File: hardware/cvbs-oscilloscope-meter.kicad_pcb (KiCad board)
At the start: 2 copper layers, 49.5 x 99.7 mm, 40 parts, among them J1 Conn_Coaxial_Power, J2 Conn_Coaxial_Power, J3 Conn_Coaxial_Power, J4 Conn_Coaxial_Power, Q1 2N3906, Q2 2N3906, Q3 2N3904, Q4 2N3904, Q5 2N3904, Q6 2N3904, U1 LM1881, U4 AD8032

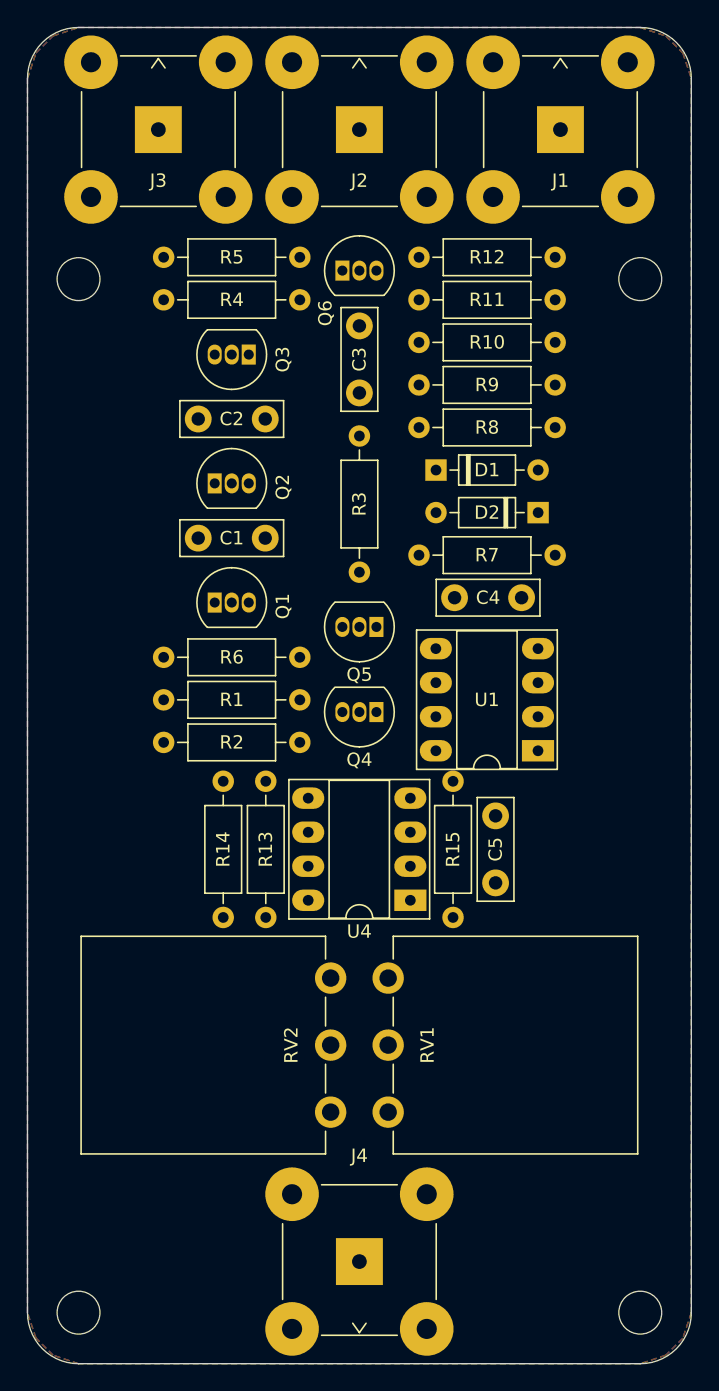
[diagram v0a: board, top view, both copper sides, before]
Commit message: Finished initial routing
Finished Routing - will need to check and revise
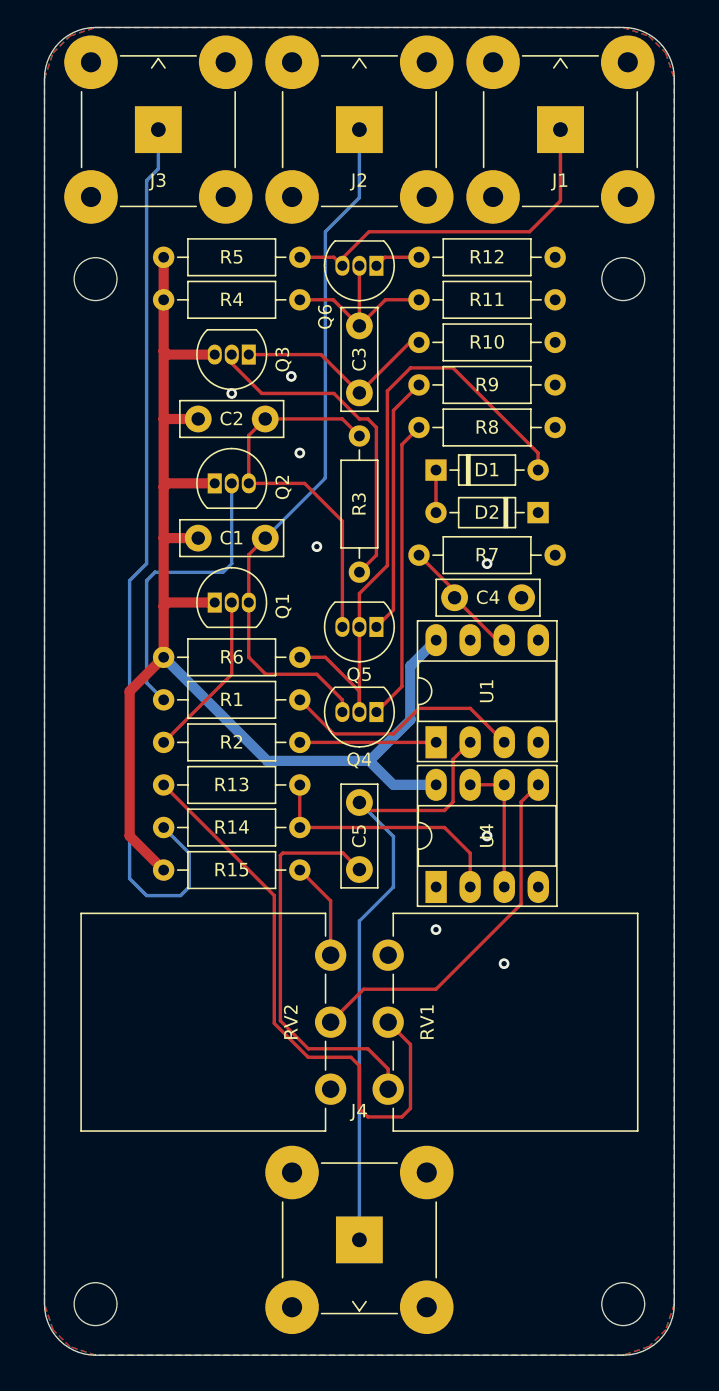
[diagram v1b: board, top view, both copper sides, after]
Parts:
- moved R15 22.6 mm to (115.4, 155.2), turned to 0 degrees
- moved C5 10.9 mm to (130.0, 155.2), turned to 90 degrees
- moved R14 8.81 mm to (125.6, 152.1), turned to 180 degrees
- moved U1 7.63 mm to (135.7, 145.7), turned to 90 degrees
- moved R13 7.62 mm to (115.4, 148.9), turned to 0 degrees
- moved Q6 2.57 mm to (131.3, 110.2), turned to 180 degrees
- moved U4 2.17 mm to (135.7, 156.5), turned to 90 degrees
- moved RV1 1.71 mm to (132.1, 171.6)
- moved RV2 1.71 mm to (127.9, 161.6)
- moved J4 1.62 mm to (130.0, 182.8)
- moved MK4 1.42 mm to (149.7, 187.6)
- moved MK3 1.42 mm to (110.3, 187.6)
- moved MK1 1.27 mm to (110.3, 111.2)
- moved MK2 1.27 mm to (149.7, 111.2)
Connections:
- U4 pad 1: (no net) -> Z
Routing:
- net +9V: track 0.00 -> 100.1 mm
- net Z: track 0.00 -> 67.2 mm
- net Y: track 0.00 -> 52.0 mm
- net Net-(D1-Pad2): track 0.00 -> 47.7 mm
- net COMP_VIDEO_IN: track 0.00 -> 47.2 mm
- net Net-(R13-Pad1): track 0.00 -> 43.5 mm
- net Net-(C5-Pad1): track 0.00 -> 29.9 mm
- net Net-(C2-Pad1): track 0.00 -> 28.9 mm
- net X: track 0.00 -> 27.4 mm
- net Net-(RV2-Pad2): track 0.00 -> 27.3 mm
- net Net-(Q3-Pad2): track 0.00 -> 24.8 mm
- net Net-(Q4-Pad1): track 0.00 -> 22.5 mm
- net Net-(Q2-Pad2): track 0.00 -> 22.3 mm
- net Net-(Q5-Pad1): track 0.00 -> 19.4 mm
- net Net-(R13-Pad2): track 0.00 -> 19.2 mm
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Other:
- board size 49.5 x 99.7 mm -> 47 x 99.1 mm
